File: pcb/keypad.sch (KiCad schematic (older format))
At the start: 8 parts, among them SW700 SW_Push, SW701 SW_Push, SW702 SW_Push, SW703 SW_Push, SW704 SW_Push, SW705 SW_Push, SW706 SW_Push, SW707 SW_Push

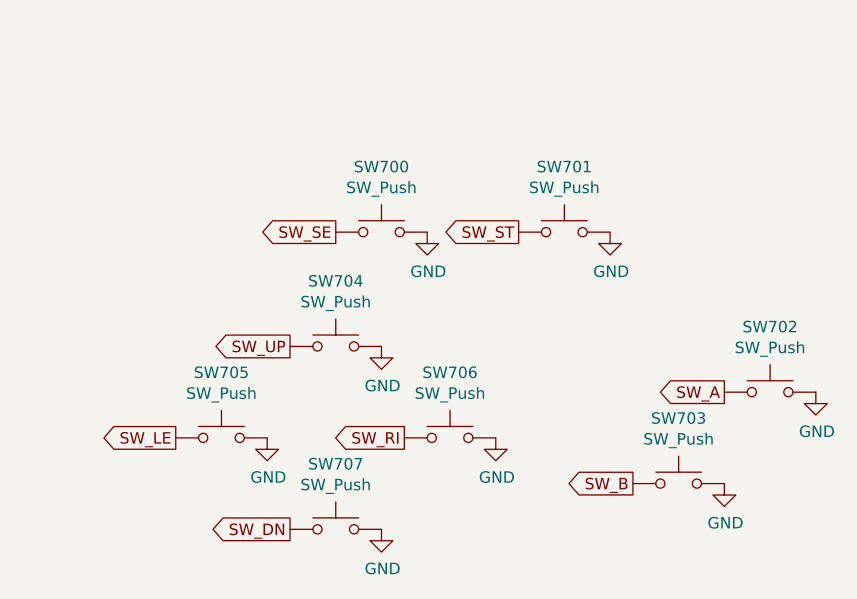
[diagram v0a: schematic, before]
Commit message: finish sch rev 0.1
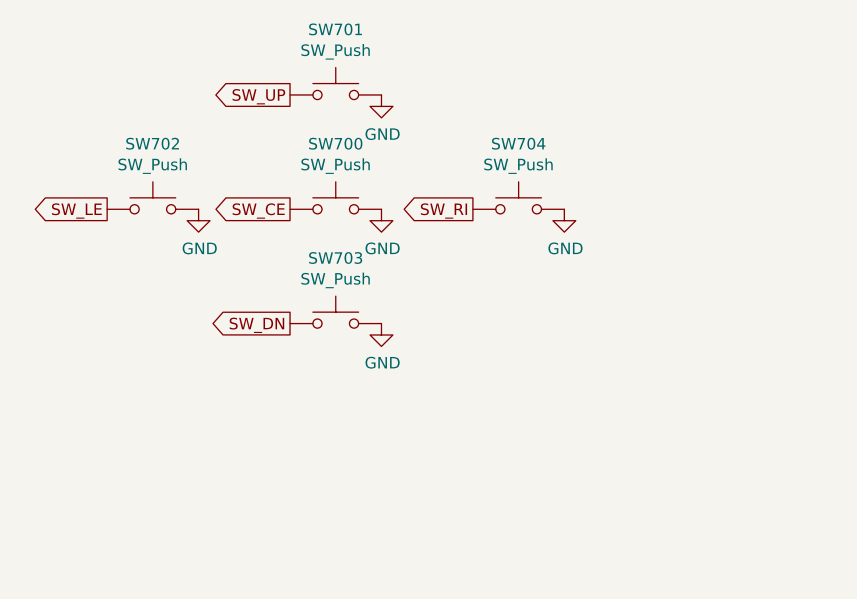
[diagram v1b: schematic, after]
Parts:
- removed SW700, SW701, SW702: SW_Push, footprints:contact, symbol Switch:SW_Push
- SW700: renamed from SW703; footprint footprints:contact -> footprints:EVQQ2
- SW701: renamed from SW704; footprint footprints:contact -> footprints:EVQQ2
- SW702: renamed from SW705; footprint footprints:contact -> footprints:EVQQ2
- SW703: renamed from SW707; footprint footprints:contact -> footprints:EVQQ2
- SW704: renamed from SW706; footprint footprints:contact -> footprints:EVQQ2
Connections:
- net SW_B renamed SW_CE
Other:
- moved on the sheet: SW700, SW701, SW702, SW703, SW704
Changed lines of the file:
@@
 EESchema Schematic File Version 4
-LIBS:pcb-cache
 EELAYER 30 0
 EELAYER END
@@
 Comment4 ""
 $EndDescr
-Text GLabel 6000 3600 0    50   Output ~ 0
-SW_ST
-Text GLabel 5500 4500 0    50   Output ~ 0
+Text GLabel 5800 3500 0    50   Output ~ 0
 SW_RI
-Text GLabel 6900 4300 0    50   Output ~ 0
-SW_A
-Text GLabel 6500 4700 0    50   Output ~ 0
-SW_B
-Text GLabel 4500 4500 0    50   Output ~ 0
+Text GLabel 5000 3500 0    50   Output ~ 0
+SW_CE
+Text GLabel 4200 3500 0    50   Output ~ 0
 SW_LE
-Text GLabel 5000 4100 0    50   Output ~ 0
+Text GLabel 5000 3000 0    50   Output ~ 0
 SW_UP
-Text GLabel 5200 3600 0    50   Output ~ 0
-SW_SE
-Text GLabel 5000 4900 0    50   Output ~ 0
+Text GLabel 5000 4000 0    50   Output ~ 0
 SW_DN
 $Comp
 L power:GND #PWR0288
 U 1 1 5D28BC76
-P 5400 4100
-F 0 "#PWR0288" H 5400 3850 50  0001 C CNN
-F 1 "GND" H 5405 3927 50  0000 C CNN
-F 2 "" H 5400 4100 50  0001 C CNN
-F 3 "" H 5400 4100 50  0001 C CNN
-	1    5400 4100
+P 5400 3000
+F 0 "#PWR0288" H 5400 2750 50  0001 C CNN
+F 1 "GND" H 5405 2827 50  0000 C CNN
+F 2 "" H 5400 3000 50  0001 C CNN
+F 3 "" H 5400 3000 50  0001 C CNN
+	1    5400 3000
 	1    0    0    -1
 $EndComp
@@
 L power:GND #PWR0287
 U 1 1 5D28B91D
-P 4900 4500
-F 0 "#PWR0287" H 4900 4250 50  0001 C CNN
-F 1 "GND" H 4905 4327 50  0000 C CNN
-F 2 "" H 4900 4500 50  0001 C CNN
-F 3 "" H 4900 4500 50  0001 C CNN
-	1    4900 4500
+P 4600 3500
+F 0 "#PWR0287" H 4600 3250 50  0001 C CNN
+F 1 "GND" H 4605 3327 50  0000 C CNN
+F 2 "" H 4600 3500 50  0001 C CNN
+F 3 "" H 4600 3500 50  0001 C CNN
+	1    4600 3500
 	1    0    0    -1
 $EndComp
@@
 L power:GND #PWR0286
 U 1 1 5D28B509
-P 5400 4900
-F 0 "#PWR0286" H 5400 4650 50  0001 C CNN
-F 1 "GND" H 5405 4727 50  0000 C CNN
-F 2 "" H 5400 4900 50  0001 C CNN
-F 3 "" H 5400 4900 50  0001 C CNN
-	1    5400 4900
+P 5400 4000
+F 0 "#PWR0286" H 5400 3750 50  0001 C CNN
+F 1 "GND" H 5405 3827 50  0000 C CNN
+F 2 "" H 5400 4000 50  0001 C CNN
+F 3 "" H 5400 4000 50  0001 C CNN
+	1    5400 4000
 	1    0    0    -1
 $EndComp
@@
 L power:GND #PWR0285
 U 1 1 5D28B128
-P 5900 4500
-F 0 "#PWR0285" H 5900 4250 50  0001 C CNN
-F 1 "GND" H 5905 4327 50  0000 C CNN
-F 2 "" H 5900 4500 50  0001 C CNN
-F 3 "" H 5900 4500 50  0001 C CNN
-	1    5900 4500
+P 6200 3500
+F 0 "#PWR0285" H 6200 3250 50  0001 C CNN
+F 1 "GND" H 6205 3327 50  0000 C CNN
+F 2 "" H 6200 3500 50  0001 C CNN
+F 3 "" H 6200 3500 50  0001 C CNN
+	1    6200 3500
 	1    0    0    -1
 $EndComp
@@
 L power:GND #PWR0284
 U 1 1 5D28AD69
-P 6900 4700
-F 0 "#PWR0284" H 6900 4450 50  0001 C CNN
-F 1 "GND" H 6905 4527 50  0000 C CNN
-F 2 "" H 6900 4700 50  0001 C CNN
-F 3 "" H 6900 4700 50  0001 C CNN
-	1    6900 4700
+P 5400 3500
+F 0 "#PWR0284" H 5400 3250 50  0001 C CNN
+F 1 "GND" H 5405 3327 50  0000 C CNN
+F 2 "" H 5400 3500 50  0001 C CNN
+F 3 "" H 5400 3500 50  0001 C CNN
+	1    5400 3500
 	1    0    0    -1
 $EndComp
 $Comp
-L power:GND #PWR0283
-U 1 1 5D28AA10
-P 7300 4300
-F 0 "#PWR0283" H 7300 4050 50  0001 C CNN
-F 1 "GND" H 7305 4127 50  0000 C CNN
-F 2 "" H 7300 4300 50  0001 C CNN
-F 3 "" H 7300 4300 50  0001 C CNN
-	1    7300 4300
+L Switch:SW_Push SW700
+U 1 1 5D27EABD
+P 5200 3500
+F 0 "SW700" H 5200 3785 50  0000 C CNN
+F 1 "SW_Push" H 5200 3694 50  0000 C CNN
+F 2 "footprints:EVQQ2" H 5200 3700 50  0001 C CNN
+F 3 "~" H 5200 3700 50  0001 C CNN
+	1    5200 3500
 	1    0    0    -1
 $EndComp
 $Comp
-L power:GND #PWR0282
-U 1 1 5D289F76
-P 5600 3600
-F 0 "#PWR0282" H 5600 3350 50  0001 C CNN
-F 1 "GND" H 5605 3427 50  0000 C CNN
-F 2 "" H 5600 3600 50  0001 C CNN
-F 3 "" H 5600 3600 50  0001 C CNN
-	1    5600 3600
+L Switch:SW_Push SW704
+U 1 1 5D27D8DE
+P 6000 3500
+F 0 "SW704" H 6000 3785 50  0000 C CNN
+F 1 "SW_Push" H 6000 3694 50  0000 C CNN
+F 2 "footprints:EVQQ2" H 6000 3700 50  0001 C CNN
+F 3 "~" H 6000 3700 50  0001 C CNN
+	1    6000 3500
 	1    0    0    -1
 $EndComp
 $Comp
-L power:GND #PWR0281
-U 1 1 5D288EE2
-P 6400 3600
-F 0 "#PWR0281" H 6400 3350 50  0001 C CNN
-F 1 "GND" H 6405 3427 50  0000 C CNN
-F 2 "" H 6400 3600 50  0001 C CNN
-F 3 "" H 6400 3600 50  0001 C CNN
-	1    6400 3600
+L Switch:SW_Push SW703
+U 1 1 5D27CCB2
+P 5200 4000
+F 0 "SW703" H 5200 4285 50  0000 C CNN
+F 1 "SW_Push" H 5200 4194 50  0000 C CNN
+F 2 "footprints:EVQQ2" H 5200 4200 50  0001 C CNN
+F 3 "~" H 5200 4200 50  0001 C CNN
+	1    5200 4000
+	1    0    0    -1
+$EndComp
+$Comp
+L Switch:SW_Push SW702
+U 1 1 5D27BD89
+P 4400 3500
+F 0 "SW702" H 4400 3785 50  0000 C CNN
+F 1 "SW_Push" H 4400 3694 50  0000 C CNN
+F 2 "footprints:EVQQ2" H 4400 3700 50  0001 C CNN
+F 3 "~" H 4400 3700 50  0001 C CNN
+	1    4400 3500
 	1    0    0    -1
 $EndComp
 $Comp
 L Switch:SW_Push SW701
-U 1 1 5D2828BB
-P 6200 3600
-F 0 "SW701" H 6200 3885 50  0000 C CNN
-F 1 "SW_Push" H 6200 3794 50  0000 C CNN
-F 2 "footprints:contact" H 6200 3800 50  0001 C CNN
-F 3 "~" H 6200 3800 50  0001 C CNN
-	1    6200 3600
+U 1 1 5D2797BD
+P 5200 3000
+F 0 "SW701" H 5200 3285 50  0000 C CNN
+F 1 "SW_Push" H 5200 3194 50  0000 C CNN
+F 2 "footprints:EVQQ2" H 5200 3200 50  0001 C CNN
+F 3 "~" H 5200 3200 50  0001 C CNN
+	1    5200 3000
 	1    0    0    -1
 $EndComp
-$Comp
-L Switch:SW_Push SW700
-U 1 1 5D281FA3
-P 5400 3600
-F 0 "SW700" H 5400 3885 50  0000 C CNN
-F 1 "SW_Push" H 5400 3794 50  0000 C CNN
-F 2 "footprints:contact" H 5400 3800 50  0001 C CNN
-F 3 "~" H 5400 3800 50  0001 C CNN
-	1    5400 3600
-	1    0    0    -1
-$EndComp
-$Comp
-L Switch:SW_Push SW703
-U 1 1 5D27EABD
-P 6700 4700
-F 0 "SW703" H 6700 4985 50  0000 C CNN
-F 1 "SW_Push" H 6700 4894 50  0000 C CNN
-F 2 "footprints:contact" H 6700 4900 50  0001 C CNN
-F 3 "~" H 6700 4900 50  0001 C CNN
-	1    6700 4700
-	1    0    0    -1
-$EndComp
-$Comp
-L Switch:SW_Push SW702
-U 1 1 5D27E22C
-P 7100 4300
-F 0 "SW702" H 7100 4585 50  0000 C CNN
-F 1 "SW_Push" H 7100 4494 50  0000 C CNN
-F 2 "footprints:contact" H 7100 4500 50  0001 C CNN
-F 3 "~" H 7100 4500 50  0001 C CNN
-	1    7100 4300
-	1    0    0    -1
-$EndComp
-$Comp
-L Switch:SW_Push SW706
-U 1 1 5D27D8DE
-P 5700 4500
-F 0 "SW706" H 5700 4785 50  0000 C CNN
-F 1 "SW_Push" H 5700 4694 50  0000 C CNN
-F 2 "footprints:contact" H 5700 4700 50  0001 C CNN
-F 3 "~" H 5700 4700 50  0001 C CNN
-	1    5700 4500
-	1    0    0    -1
-$EndComp
-$Comp
-L Switch:SW_Push SW707
-U 1 1 5D27CCB2
-P 5200 4900
-F 0 "SW707" H 5200 5185 50  0000 C CNN
-F 1 "SW_Push" H 5200 5094 50  0000 C CNN
-F 2 "footprints:contact" H 5200 5100 50  0001 C CNN
-F 3 "~" H 5200 5100 50  0001 C CNN
-	1    5200 4900
-	1    0    0    -1
-$EndComp
-$Comp
-L Switch:SW_Push SW705
-U 1 1 5D27BD89
-P 4700 4500
-F 0 "SW705" H 4700 4785 50  0000 C CNN
-F 1 "SW_Push" H 4700 4694 50  0000 C CNN
-F 2 "footprints:contact" H 4700 4700 50  0001 C CNN
-F 3 "~" H 4700 4700 50  0001 C CNN
-	1    4700 4500
-	1    0    0    -1
-$EndComp
-$Comp
-L Switch:SW_Push SW704
-U 1 1 5D2797BD
-P 5200 4100
-F 0 "SW704" H 5200 4385 50  0000 C CNN
-F 1 "SW_Push" H 5200 4294 50  0000 C CNN
-F 2 "footprints:contact" H 5200 4300 50  0001 C CNN
-F 3 "~" H 5200 4300 50  0001 C CNN
-	1    5200 4100
-	1    0    0    -1
-$EndComp
